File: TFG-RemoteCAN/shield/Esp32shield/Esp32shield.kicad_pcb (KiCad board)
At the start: 2 copper layers, 8 parts, among them J1 PINS_1, J2 PINS_2, J3 Screw_Terminal_01x02, J4 Conn_01x04, J5 Conn_01x01, J6 Conn_01x01, J7 Conn_01x01, J8 Conn_01x01

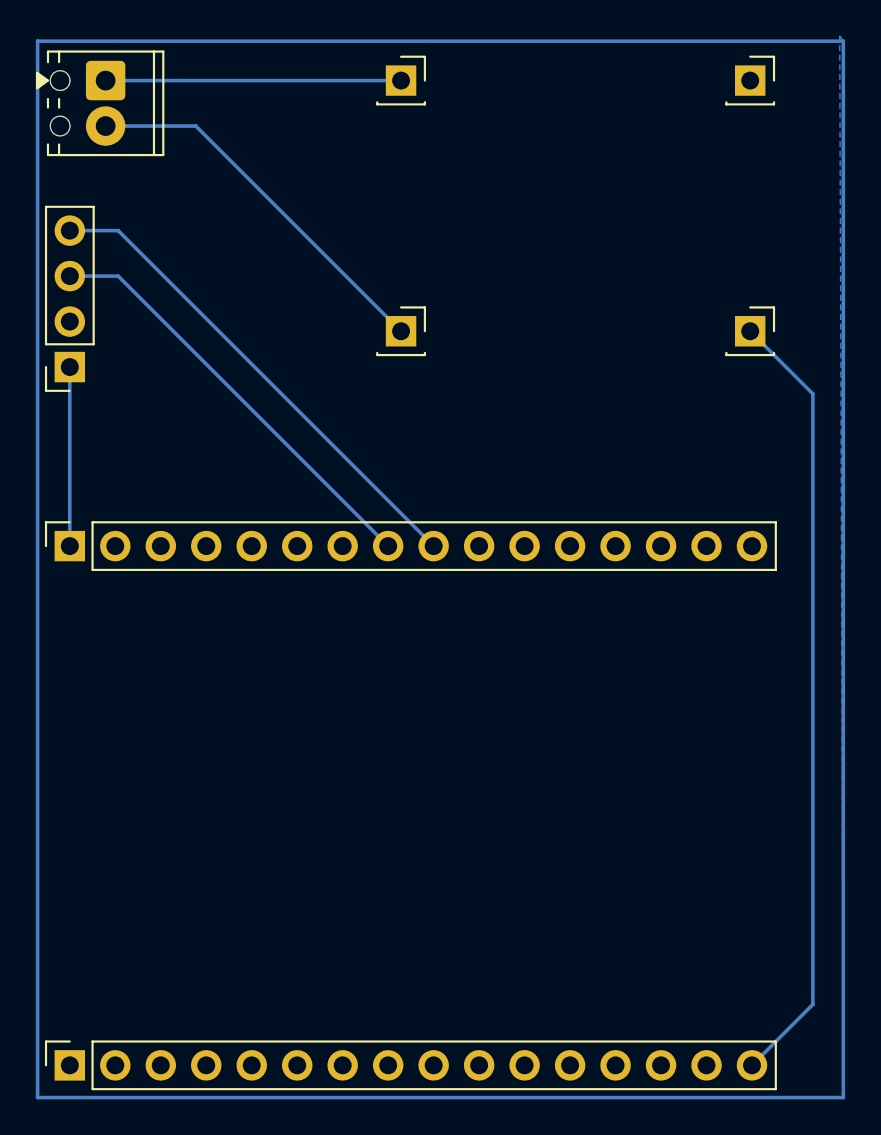
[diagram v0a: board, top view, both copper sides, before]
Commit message: Versió 1.1
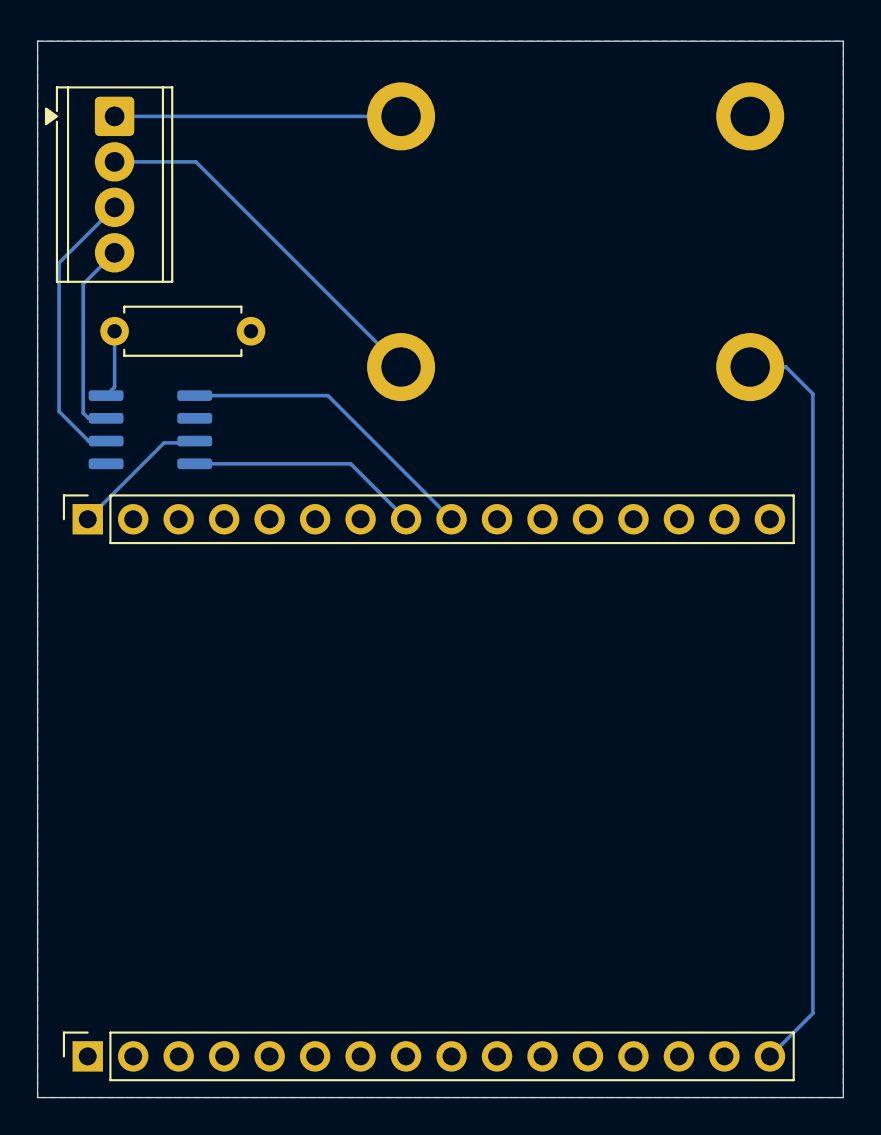
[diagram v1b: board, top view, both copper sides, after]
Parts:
- removed J7, J8: Conn_01x01, Connector_PinSocket_2.54mm:PinSocket_1x01_P2.54mm_Vertical
- added J9: Screw_Terminal_01x04, TerminalBlock_Phoenix:TerminalBlock_Phoenix_MPT-0,5-4-2.54_1x04_P2.54mm_Horizontal, F.Cu at (44.0, 32.0)
- added R1: 10000, Resistor_THT:R_Axial_DIN0207_L6.3mm_D2.5mm_P7.62mm_Horizontal, F.Cu at (44.0, 44.0)
- added U1: SN65HVD230, Package_SO:SOIC-8_3.9x4.9mm_P1.27mm, B.Cu at (46.0, 49.5)
- J3: value Screw_Terminal_01x02 -> Conn_01x01_Socket; footprint TerminalBlock_Phoenix:TerminalBlock_Phoenix_MPT-0,5-2-2.54_1x02_P2.54mm_Horizontal -> MountingHole:MountingHole_2.2mm_M2_DIN965_Pad
- J4: value Conn_01x04 -> Conn_01x01_Socket; footprint Connector_PinSocket_2.54mm:PinSocket_1x04_P2.54mm_Vertical -> MountingHole:MountingHole_2.2mm_M2_DIN965_Pad
- J5, J6: value Conn_01x01 -> Conn_01x01_Socket; footprint Connector_PinSocket_2.54mm:PinSocket_1x01_P2.54mm_Vertical -> MountingHole:MountingHole_2.2mm_M2_DIN965_Pad
- moved J4 23.2 mm to (60.0, 32.0), turned to 0 degrees
- moved J3 23.0 mm to (60.0, 46.0), turned to 0 degrees
- moved J5 19.6 mm to (79.5, 46.0)
- moved J6 19.6 mm to (79.5, 32.0)
- moved J1 1.80 mm to (42.5, 54.5)
- moved J2 1.12 mm to (42.5, 84.5)
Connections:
- J3 pad 1: GNDBAT -> +12V
- J4 pad 1: +3.3V -> GNDBAT
- J5 pad 1: +12V -> VIN
- J6 pad 1: GNDBAT -> GND
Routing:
- net CAN_L: track 0.00 -> 16.0 mm
- net CAN_H: track 0.00 -> 11.1 mm
- net RXD: track 24.0 -> 13.1 mm
- net TXD: track 27.6 -> 17.2 mm
- net Net-(U1-Rs): track 0.00 -> 3.79 mm
- net VIN: track 43.9 -> 42.1 mm
- net +3.3V: track 10.0 -> 8.59 mm
- net GNDBAT: track 16.5 -> 17.1 mm
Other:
- board outline added: 45 x 59 mm
